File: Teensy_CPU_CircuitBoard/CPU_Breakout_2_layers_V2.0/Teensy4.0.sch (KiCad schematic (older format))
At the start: 11 parts, among them SW1 SW_Push, SW2 SW_Push, T4 BreakoutBoardTeensy_Teensy_pi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, U1 S8211-46R

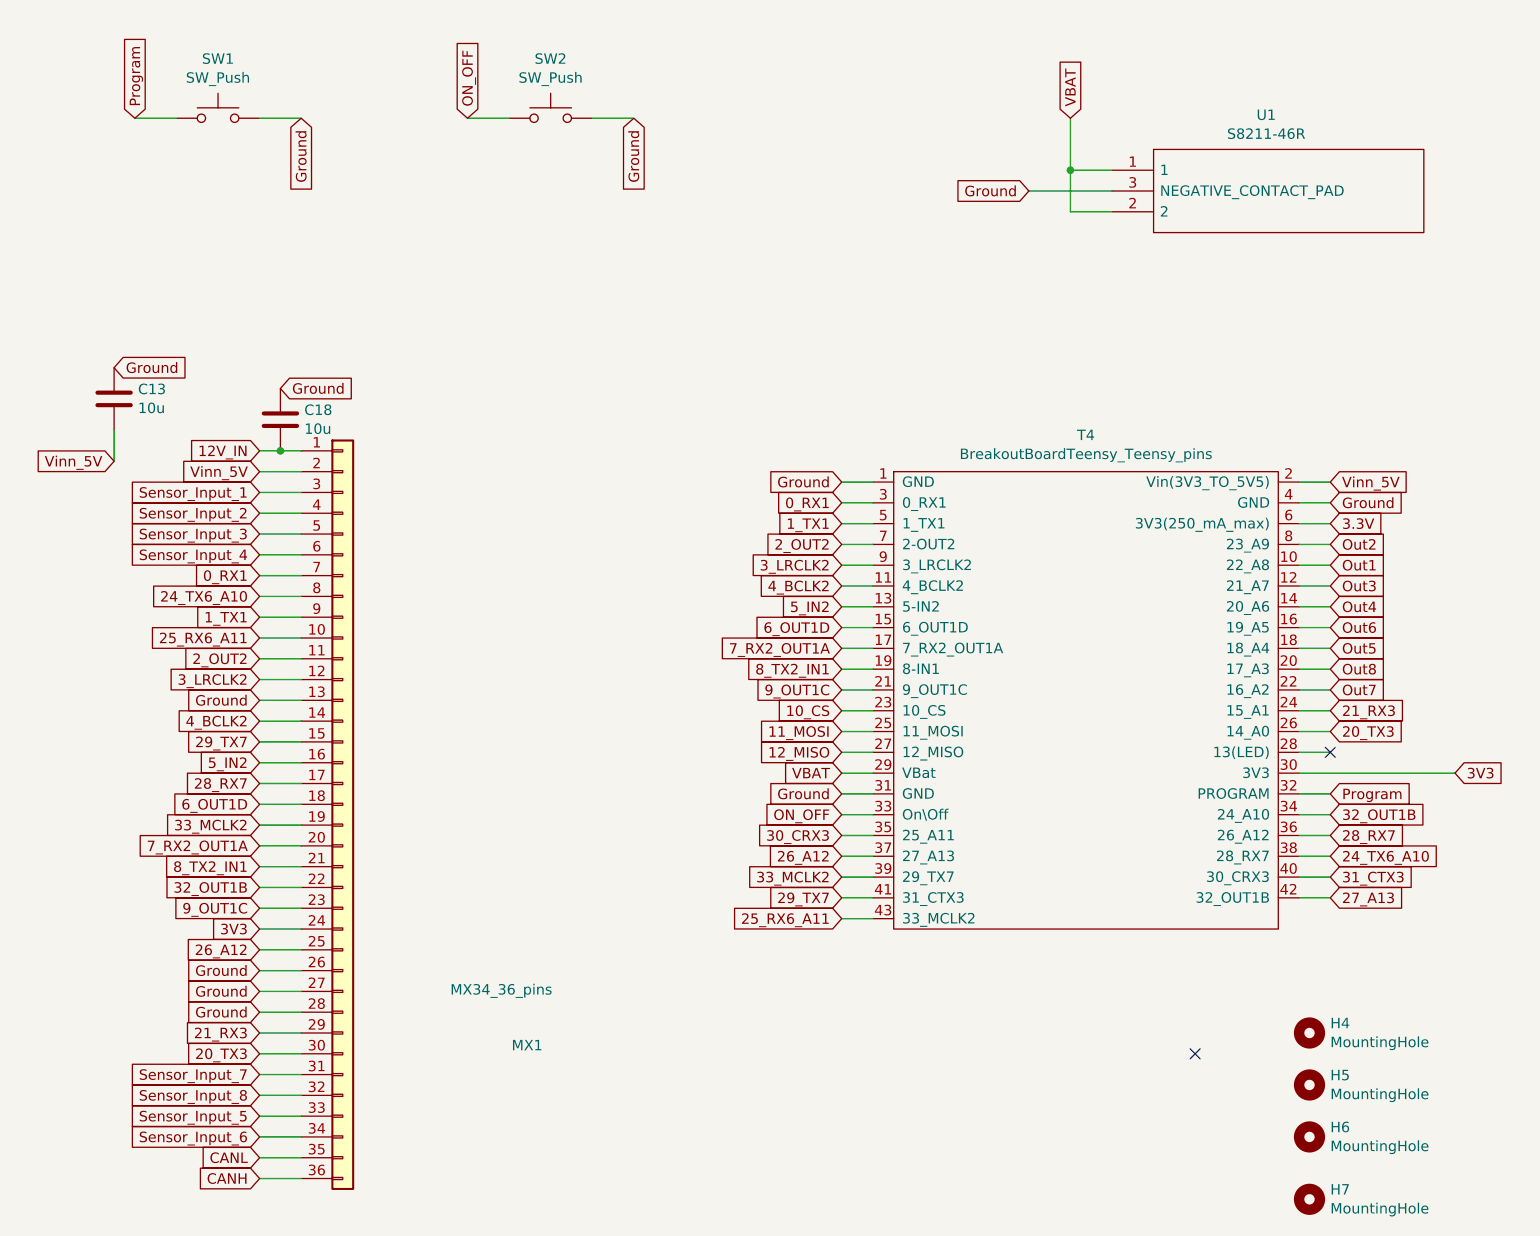
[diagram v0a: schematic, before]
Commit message: Start of V3 STM32
Imported symbols/footprints ...
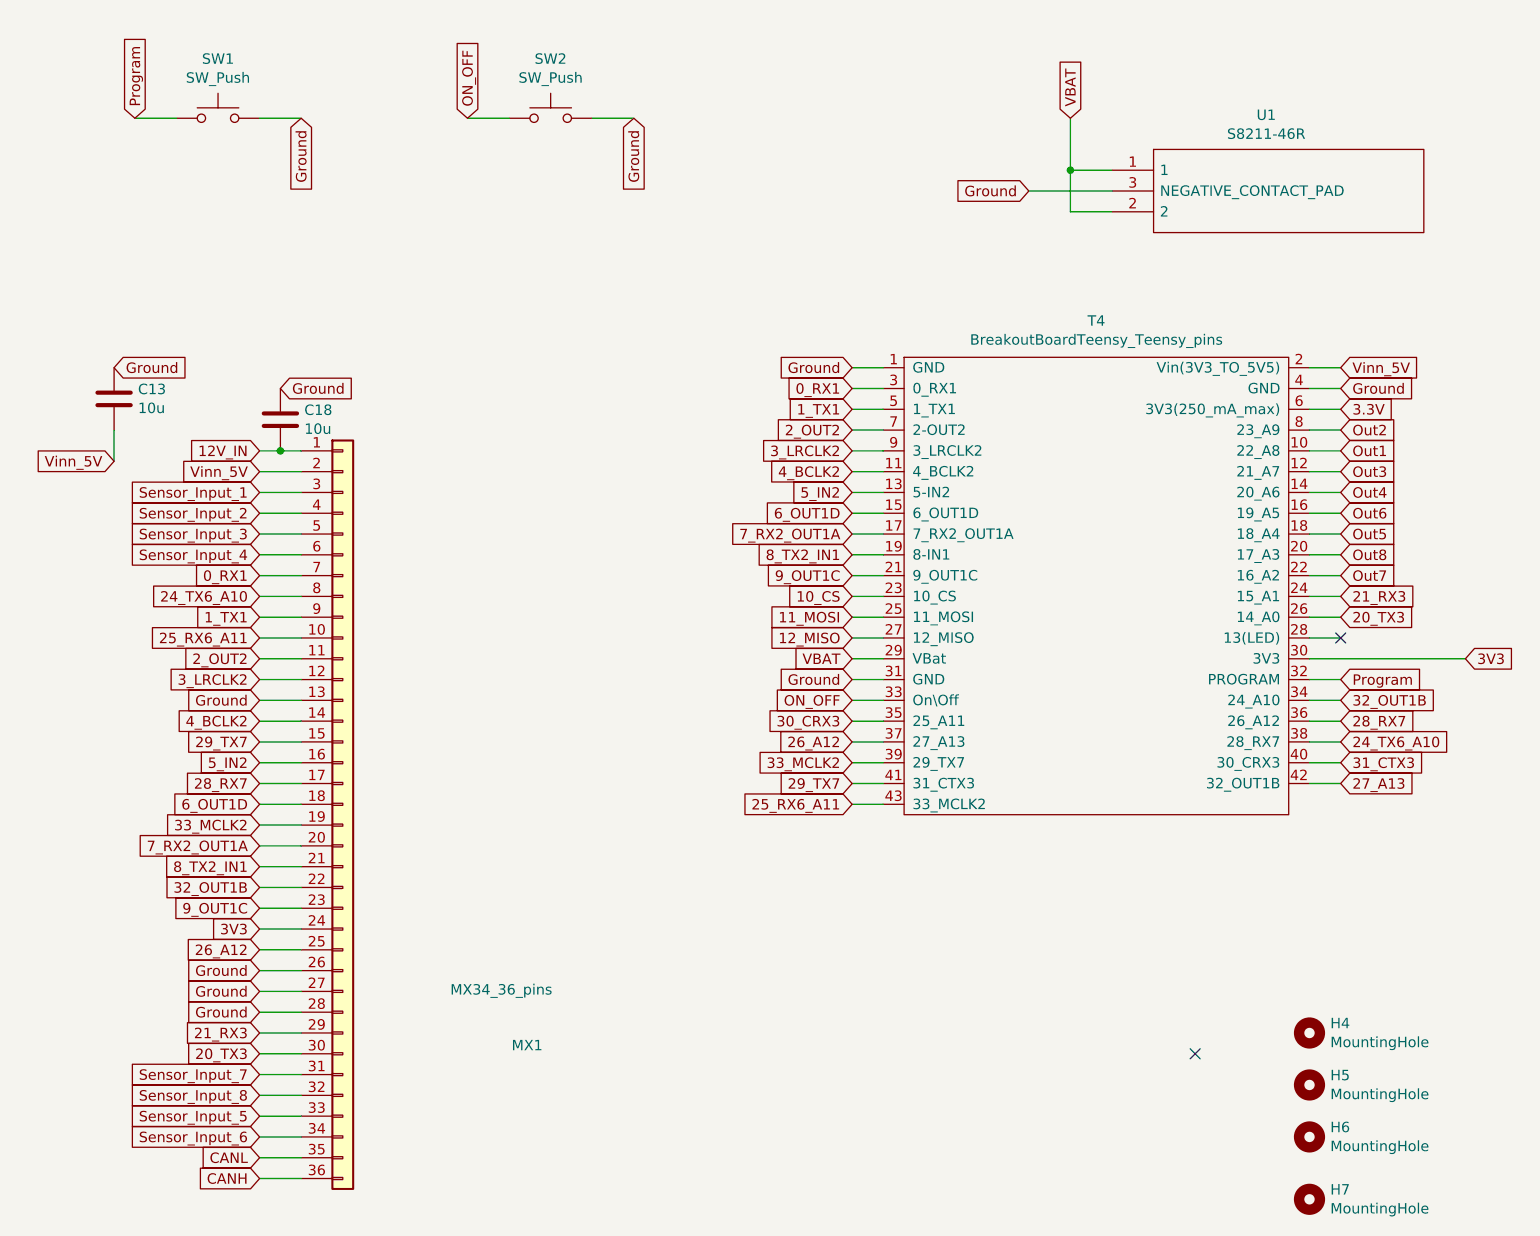
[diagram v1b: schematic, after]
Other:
- moved on the sheet: T4
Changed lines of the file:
@@
 $Descr A4 11693 8268
 encoding utf-8
-Sheet 6 6
+Sheet 5 5
 Title ""
 Date ""
@@
 Comment4 ""
 $EndDescr
-Text GLabel 6800 4250 0    50   Input ~ 0
+Text GLabel 6850 3700 0    50   Input ~ 0
 Ground
-Text GLabel 9150 2850 2    50   Input ~ 0
+Text GLabel 9200 2300 2    50   Input ~ 0
 Ground
-Text GLabel 9150 3250 2    50   Input ~ 0
+Text GLabel 9200 2700 2    50   Input ~ 0
 Out3
-Text GLabel 9150 3150 2    50   Input ~ 0
+Text GLabel 9200 2600 2    50   Input ~ 0
 Out1
-Text GLabel 9150 3050 2    50   Input ~ 0
+Text GLabel 9200 2500 2    50   Input ~ 0
 Out2
-Text GLabel 9150 3350 2    50   Input ~ 0
+Text GLabel 9200 2800 2    50   Input ~ 0
 Out4
-Text GLabel 6800 4550 0    50   Input ~ 0
+Text GLabel 6850 4000 0    50   Input ~ 0
 26_A12
-Text GLabel 9150 4550 2    50   Input ~ 0
+Text GLabel 9200 4000 2    50   Input ~ 0
 24_TX6_A10
-Text GLabel 9750 4150 2    50   Input ~ 0
+Text GLabel 9800 3600 2    50   Input ~ 0
 3V3
-Text GLabel 9150 2950 2    50   Input ~ 0
+Text GLabel 9200 2400 2    50   Input ~ 0
 3.3V
-Text GLabel 9150 2750 2    50   Input ~ 0
+Text GLabel 9200 2200 2    50   Input ~ 0
 Vinn_5V
-Text GLabel 9150 3850 2    50   Input ~ 0
+Text GLabel 9200 3300 2    50   Input ~ 0
 21_RX3
-Text GLabel 9150 3950 2    50   Input ~ 0
+Text GLabel 9200 3400 2    50   Input ~ 0
 20_TX3
-Text GLabel 9150 4450 2    50   Input ~ 0
+Text GLabel 9200 3900 2    50   Input ~ 0
 28_RX7
-Text GLabel 6800 4450 0    50   Input ~ 0
+Text GLabel 6850 3900 0    50   Input ~ 0
 30_CRX3
-Text GLabel 9150 4350 2    50   Input ~ 0
+Text GLabel 9200 3800 2    50   Input ~ 0
 32_OUT1B
-Text GLabel 6800 3950 0    50   Input ~ 0
+Text GLabel 6850 3400 0    50   Input ~ 0
 11_MOSI
-Text GLabel 6800 3850 0    50   Input ~ 0
+Text GLabel 6850 3300 0    50   Input ~ 0
 10_CS
-Text GLabel 6800 4650 0    50   Input ~ 0
+Text GLabel 6850 4100 0    50   Input ~ 0
 33_MCLK2
-Text GLabel 9150 4650 2    50   Input ~ 0
+Text GLabel 9200 4100 2    50   Input ~ 0
 31_CTX3
-Text GLabel 6800 4750 0    50   Input ~ 0
+Text GLabel 6850 4200 0    50   Input ~ 0
 29_TX7
-Text GLabel 9150 4750 2    50   Input ~ 0
+Text GLabel 9200 4200 2    50   Input ~ 0
 27_A13
-Text GLabel 6800 4850 0    50   Input ~ 0
+Text GLabel 6850 4300 0    50   Input ~ 0
 25_RX6_A11
-Text GLabel 6800 3750 0    50   Input ~ 0
+Text GLabel 6850 3200 0    50   Input ~ 0
 9_OUT1C
-Text GLabel 6800 3650 0    50   Input ~ 0
+Text GLabel 6850 3100 0    50   Input ~ 0
 8_TX2_IN1
-Text GLabel 6800 3550 0    50   Input ~ 0
+Text GLabel 6850 3000 0    50   Input ~ 0
 7_RX2_OUT1A
-Text GLabel 6800 3450 0    50   Input ~ 0
+Text GLabel 6850 2900 0    50   Input ~ 0
 6_OUT1D
-Text GLabel 6800 3350 0    50   Input ~ 0
+Text GLabel 6850 2800 0    50   Input ~ 0
 5_IN2
-Text GLabel 6800 3250 0    50   Input ~ 0
+Text GLabel 6850 2700 0    50   Input ~ 0
 4_BCLK2
-Text GLabel 6800 3150 0    50   Input ~ 0
+Text GLabel 6850 2600 0    50   Input ~ 0
 3_LRCLK2
-Text GLabel 6800 3050 0    50   Input ~ 0
+Text GLabel 6850 2500 0    50   Input ~ 0
 2_OUT2
-Text GLabel 6800 2950 0    50   Input ~ 0
+Text GLabel 6850 2400 0    50   Input ~ 0
 1_TX1
-Text GLabel 6800 2850 0    50   Input ~ 0
+Text GLabel 6850 2300 0    50   Input ~ 0
 0_RX1
-Text GLabel 6800 4050 0    50   Input ~ 0
+Text GLabel 6850 3500 0    50   Input ~ 0
 12_MISO
-Text GLabel 6800 4150 0    50   Input ~ 0
+Text GLabel 6850 3600 0    50   Input ~ 0
 VBAT
-Text GLabel 6800 4350 0    50   Input ~ 0
+Text GLabel 6850 3800 0    50   Input ~ 0
 ON_OFF
-Text GLabel 6800 2750 0    50   Input ~ 0
+Text GLabel 6850 2200 0    50   Input ~ 0
 Ground
 Text GLabel 5800 1000 3    50   Input ~ 0
@@
 VBAT
 $Bitmap
-Pos 1600 1500
+Pos 1550 1700
 Scale 1.000000
 Data
@@
 Text GLabel 4000 5800 0    50   Input ~ 0
 Sensor_Input_5
-Text GLabel 9150 3750 2    50   Input ~ 0
+Text GLabel 9200 3200 2    50   Input ~ 0
 Out7
-Text GLabel 9150 3550 2    50   Input ~ 0
+Text GLabel 9200 3000 2    50   Input ~ 0
 Out5
-Text GLabel 9150 3450 2    50   Input ~ 0
+Text GLabel 9200 2900 2    50   Input ~ 0
 Out6
-Text GLabel 9150 3650 2    50   Input ~ 0
+Text GLabel 9200 3100 2    50   Input ~ 0
 Out8
 Text GLabel 4000 5100 0    50   Input ~ 0
@@
 L teensy4_header_breakout-cache:Teensy_pins T4
 U 1 1 5E646C7B
-P 7400 3450
-F 0 "T4" H 7975 4375 50  0000 C CNN
-F 1 "BreakoutBoardTeensy_Teensy_pins" H 7975 4284 50  0000 C CNN
-F 2 "Teensy_Footprint_Library:Teensy_40_footprint" H 8700 3450 50  0001 C CNN
-F 3 "" H 8700 3450 50  0001 C CNN
-	1    7400 3450
+P 7450 2900
+F 0 "T4" H 8025 3825 50  0000 C CNN
+F 1 "BreakoutBoardTeensy_Teensy_pins" H 8025 3734 50  0000 C CNN
+F 2 "Teensy_Footprint_Library:Teensy_40_footprint" H 8750 2900 50  0001 C CNN
+F 3 "" H 8750 2900 50  0001 C CNN
+	1    7450 2900
 	1    0    0    -1
 $EndComp
 Wire Wire Line
-	6950 2750 6800 2750
+	7000 2200 6850 2200
 Wire Wire Line
-	6950 4850 6800 4850
+	7000 4300 6850 4300
 Wire Wire Line
-	6950 4750 6800 4750
+	7000 4200 6850 4200
 Wire Wire Line
-	6950 4650 6800 4650
+	7000 4100 6850 4100
 Wire Wire Line
-	6950 4550 6800 4550
+	7000 4000 6850 4000
 Wire Wire Line
-	6950 4450 6800 4450
+	7000 3900 6850 3900
 Wire Wire Line
-	6950 4350 6800 4350
+	7000 3800 6850 3800
 Wire Wire Line
-	6950 4250 6800 4250
+	7000 3700 6850 3700
 Wire Wire Line
-	6950 4150 6800 4150
+	7000 3600 6850 3600
 Wire Wire Line
-	6950 4050 6800 4050
+	7000 3500 6850 3500
 Wire Wire Line
-	6950 3950 6800 3950
+	7000 3400 6850 3400
 Wire Wire Line
-	6950 3850 6800 3850
+	7000 3300 6850 3300
 Wire Wire Line
-	6950 3750 6800 3750
+	7000 3200 6850 3200
 Wire Wire Line
-	6950 3650 6800 3650
+	7000 3100 6850 3100
 Wire Wire Line
-	6950 3550 6800 3550
+	7000 3000 6850 3000
 Wire Wire Line
-	6950 3450 6800 3450
+	7000 2900 6850 2900
 Wire Wire Line
-	6950 3350 6800 3350
+	7000 2800 6850 2800
 Wire Wire Line
-	6950 3250 6800 3250
+	7000 2700 6850 2700
 Wire Wire Line
-	6950 3150 6800 3150
+	7000 2600 6850 2600
 Wire Wire Line
-	6950 3050 6800 3050
+	7000 2500 6850 2500
 Wire Wire Line
-	6950 2950 6800 2950
+	7000 2400 6850 2400
 Wire Wire Line
-	6950 2850 6800 2850
+	7000 2300 6850 2300
 Wire Wire Line
-	9000 2750 9150 2750
+	9050 2200 9200 2200
 Wire Wire Line
-	9000 2850 9150 2850
+	9050 2300 9200 2300
 Wire Wire Line
-	9000 2950 9150 2950
+	9050 2400 9200 2400
 Wire Wire Line
-	9000 3050 9150 3050
+	9050 2500 9200 2500
 Wire Wire Line
-	9000 3150 9150 3150
+	9050 2600 9200 2600
 Wire Wire Line
-	9000 3250 9150 3250
+	9050 2700 9200 2700
 Wire Wire Line
-	9000 3350 9150 3350
+	9050 2800 9200 2800
 Wire Wire Line
-	9000 3450 9150 3450
+	9050 2900 9200 2900
 Wire Wire Line
-	9000 3550 9150 3550
+	9050 3000 9200 3000
 Wire Wire Line
-	9000 3650 9150 3650
+	9050 3100 9200 3100
 Wire Wire Line
-	9000 3750 9150 3750
+	9050 3200 9200 3200
 Wire Wire Line
-	9000 3850 9150 3850
+	9050 3300 9200 3300
 Wire Wire Line
-	9000 3950 9150 3950
+	9050 3400 9200 3400
 Wire Wire Line
-	9000 4050 9150 4050
+	9050 3500 9200 3500
 Wire Wire Line
-	9000 4150 9750 4150
+	9050 3600 9800 3600
 Wire Wire Line
-	9000 4250 9150 4250
+	9050 3700 9200 3700
 Wire Wire Line
-	9000 4350 9150 4350
+	9050 3800 9200 3800
 Wire Wire Line
-	9000 4450 9150 4450
+	9050 3900 9200 3900
 Wire Wire Line
-	9000 4550 9150 4550
+	9050 4000 9200 4000
 Wire Wire Line
-	9000 4650 9150 4650
+	9050 4100 9200 4100
 Wire Wire Line
-	9000 4750 9150 4750
+	9050 4200 9200 4200
 Wire Wire Line
 	4200 2600 4100 2600
@@
 Wire Wire Line
 	3600 1000 3400 1000
-Text GLabel 9150 4250 2    50   Input ~ 0
+Text GLabel 9200 3700 2    50   Input ~ 0
 Program
 Text GLabel 3400 1000 1    50   Input ~ 0
@@
 Wire Wire Line
 	3300 2500 3300 2650
-NoConn ~ 9150 4050
+NoConn ~ 9200 3500
 NoConn ~ 8500 5500
 Text GLabel 4000 3800 0    50   Input ~ 0
